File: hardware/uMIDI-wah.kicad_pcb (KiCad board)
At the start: 2 copper layers, 50 x 24 mm, 45 parts, among them Q1 BSS138, U1 TL071CPSR, X1 9V, X2 uMIDI, X3 Input, X4 Output

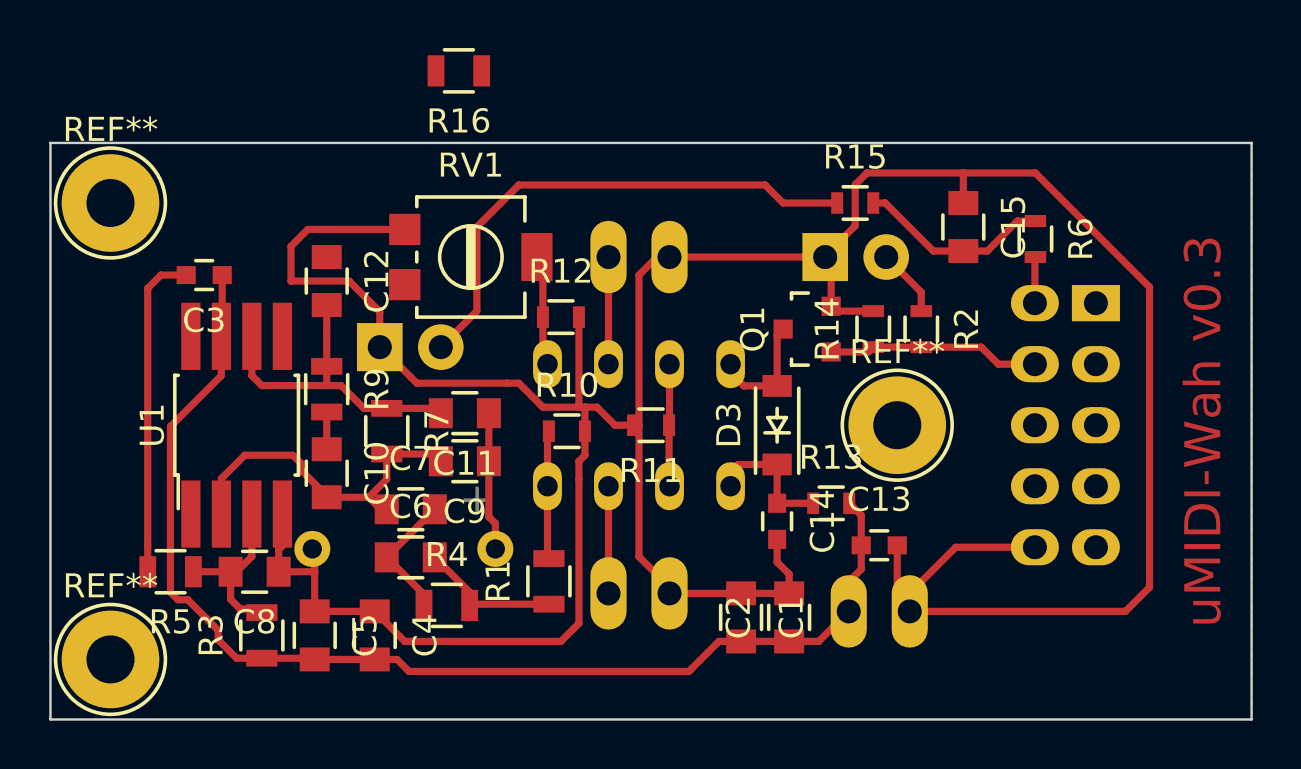
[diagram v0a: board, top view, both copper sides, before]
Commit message: Place and route
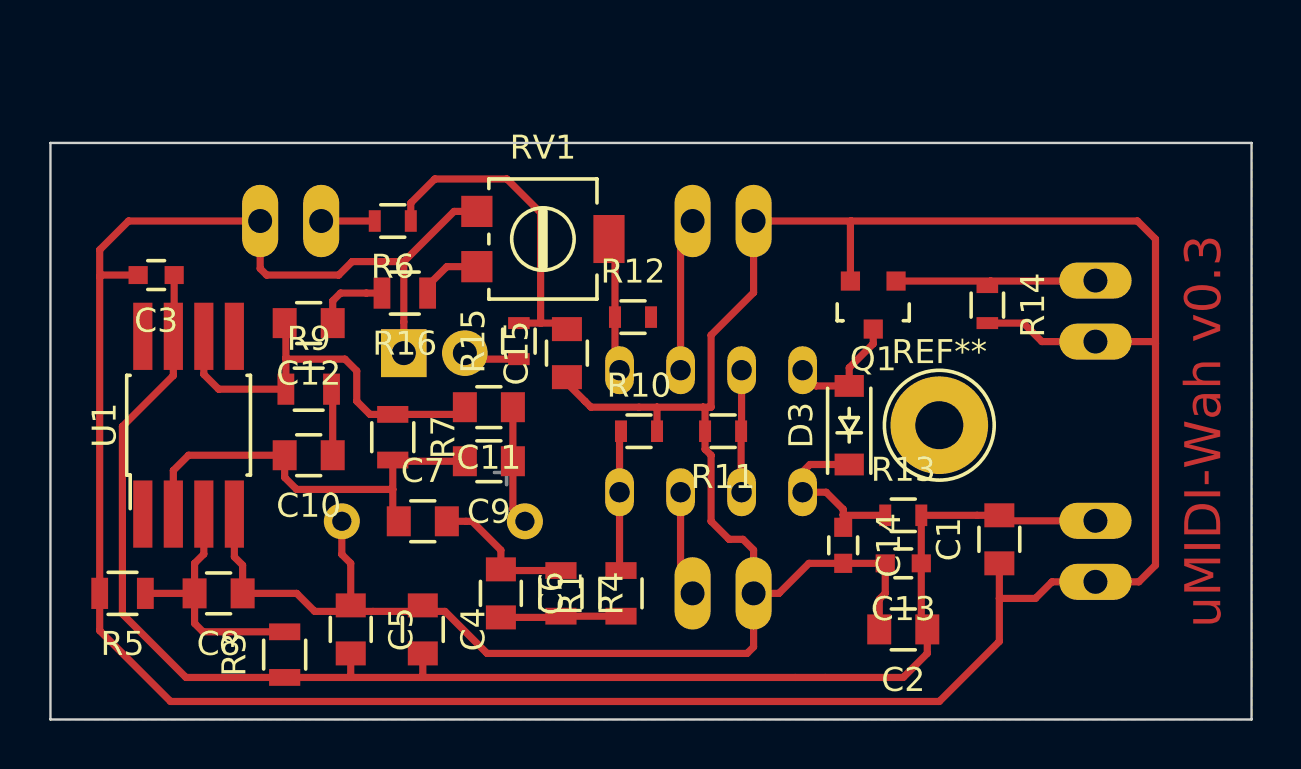
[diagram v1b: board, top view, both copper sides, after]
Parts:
- removed D1: LED, LEDs:LED-5MM
- removed R2: 82, Resistors_SMD:R_0603
- removed the REF** at (182.5, 147.5)
- removed the REF** at (182.5, 128.5)
- added X5: Enable, Connect:PINHEAD1-2, B.Cu at (223.5, 133.0)
- X2: value uMIDI -> PWM; footprint uMIDI-wah:VASCH5x2_diy-pcb -> Connect:PINHEAD1-2
- moved X2 33.4 mm to (190.0, 129.2), turned to 0 degrees
- moved R6 26.8 mm to (194.2, 129.2), turned to 180 degrees
- moved C15 17.3 mm to (201.5, 134.8), turned to 90 degrees
- moved R15 15.1 mm to (199.5, 134.2), turned to 90 degrees
- moved C1 11.2 mm to (219.5, 142.5), turned to 90 degrees
- moved R16 9.52 mm to (194.8, 132.2)
- moved X1 9.34 mm to (223.5, 143.0), turned to 90 degrees
- moved R14 4.85 mm to (219.0, 132.8), turned to 270 degrees
- moved C2 4.78 mm to (215.5, 146.2), turned to 180 degrees
- moved R4 4.78 mm to (201.2, 144.8), turned to 270 degrees
- moved C6 4.04 mm to (198.8, 144.8), turned to 270 degrees
- moved X4 3.81 mm to (208.0, 129.2)
- moved X3 3.50 mm to (208.0, 144.8)
- moved RV1 3.09 mm to (200.5, 130.0)
- moved R1 3.04 mm to (203.8, 144.8)
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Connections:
- X2 pad 1: (no net) -> GND
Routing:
- net GND: track 155.9 -> 198.5 mm
- net Net-(D2-Pad2): track 21.7 -> 2.35 mm
- net +9V: track 51.7 -> 66.9 mm
- net Net-(C15-Pad2): track 8.10 -> 13.8 mm
- net Net-(C11-Pad2): track 13.0 -> 16.9 mm
- net Net-(C10-Pad2): track 13.2 -> 17.0 mm
- net Net-(C8-Pad2): track 9.56 -> 13.1 mm
- net Net-(C12-Pad1): track 0.00 -> 3.11 mm
- net Net-(D1-Pad2): track 2.85 -> 0.00 mm
- net Net-(R16-Pad1): track 0.00 -> 2.68 mm
- net /True bypass/Loop_Out: track 4.46 -> 6.42 mm
- net /True bypass/relais_p: track 5.78 -> 7.16 mm
- net Net-(C10-Pad1): track 1.55 -> 2.77 mm
- net Net-(C6-Pad2): track 5.92 -> 5.02 mm
- net Net-(C11-Pad1): track 5.76 -> 5.09 mm
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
